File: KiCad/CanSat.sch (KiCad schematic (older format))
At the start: 0 parts

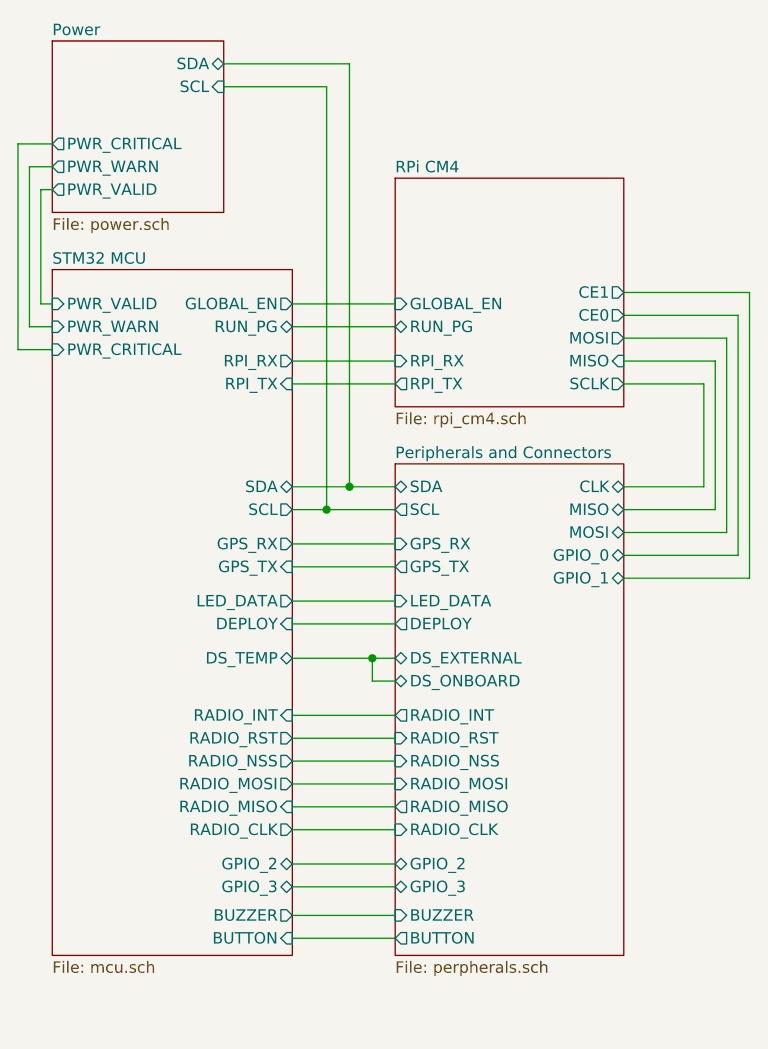
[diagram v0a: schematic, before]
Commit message: Dirty production PCBs commit
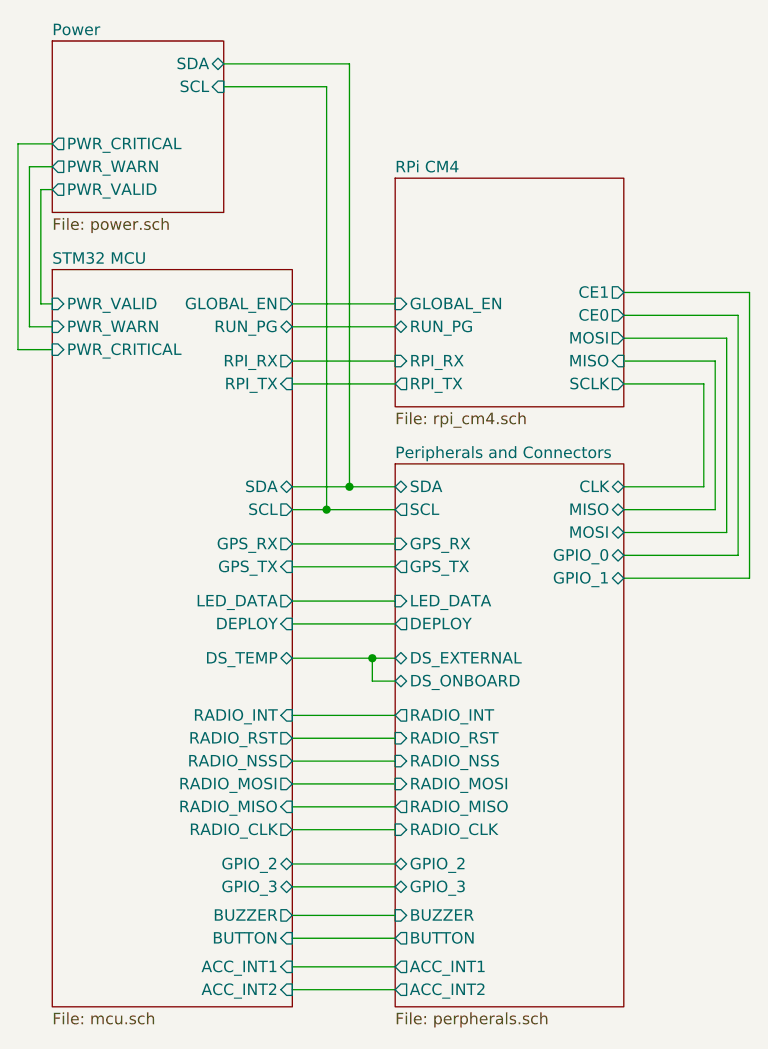
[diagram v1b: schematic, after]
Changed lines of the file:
@@
 	3500 3000 3050 3000
 $Sheet
-S 2000 2500 1050 3000
+S 2000 2500 1050 3225
 U 5FCA62D1
 F0 "STM32 MCU" 50
@@
 F24 "BUZZER" O R 3050 5325 50
 F25 "BUTTON" I R 3050 5425 50
+F26 "ACC_INT2" I R 3050 5650 50
+F27 "ACC_INT1" I R 3050 5550 50
 $EndSheet
 Wire Wire Line
@@
 F10 "CE1" O R 4500 2600 50
 $EndSheet
+Wire Wire Line
+	3500 5325 3050 5325
+Wire Wire Line
+	3500 5425 3050 5425
 $Sheet
-S 3500 3350 1000 2150
+S 3500 3350 1000 2375
 U 5FCA658C
 F0 "Peripherals and Connectors" 50
@@
 F23 "BUZZER" I L 3500 5325 50
 F24 "BUTTON" O L 3500 5425 50
+F25 "ACC_INT1" O L 3500 5550 50
+F26 "ACC_INT2" O L 3500 5650 50
 $EndSheet
 Wire Wire Line
-	3500 5325 3050 5325
+	3050 5550 3500 5550
 Wire Wire Line
-	3500 5425 3050 5425
+	3500 5650 3050 5650
 $EndSCHEMATC
